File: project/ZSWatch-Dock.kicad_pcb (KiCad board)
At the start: 2 copper layers, 52 x 52 mm, 44 parts, among them IC1 XC9265C181MR-G, IC2 MIC5219-3.3YM5, IC3 NTS0104GU12, IC4 STM32F072CBT6, Q1 BSH205G2AR, SW2 CHARGE, X1 WATCH, X3 DEBUG, X4 USB4105-GF-A

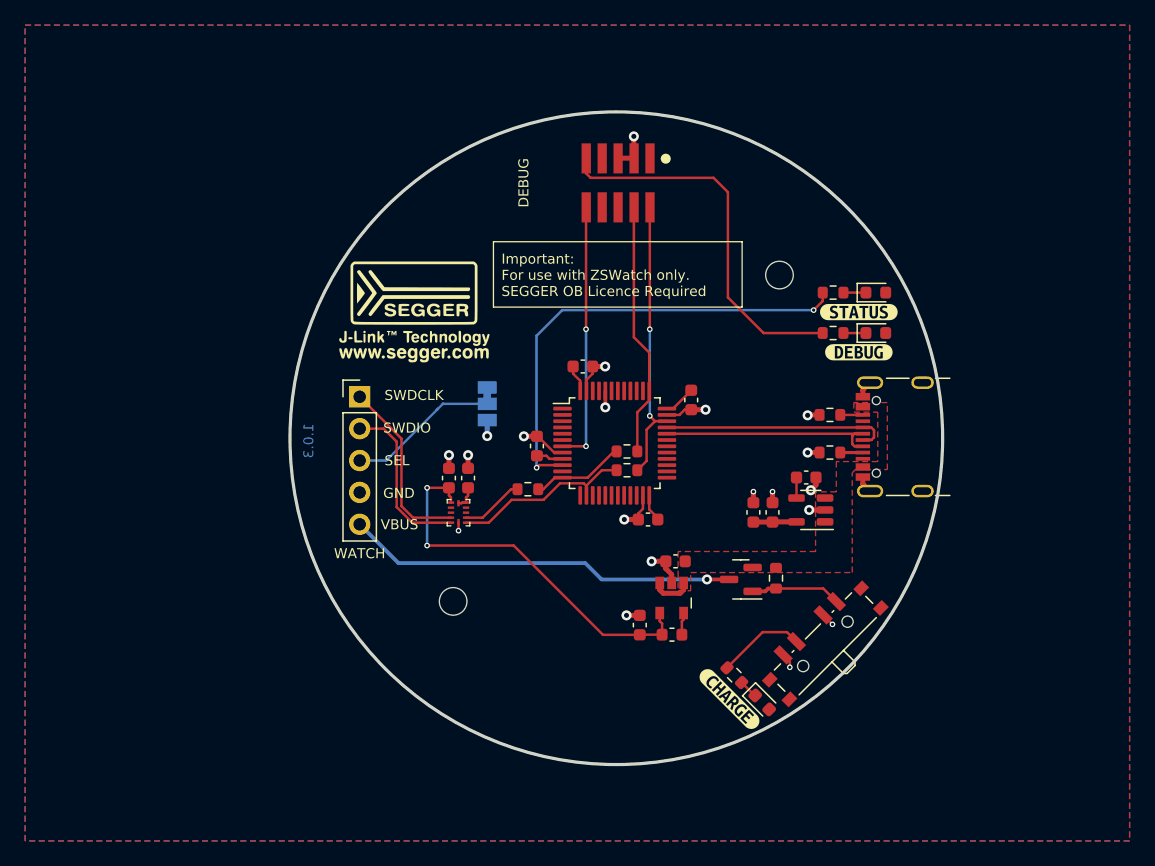
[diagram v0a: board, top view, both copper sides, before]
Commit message: Add second USB interface, rename variants
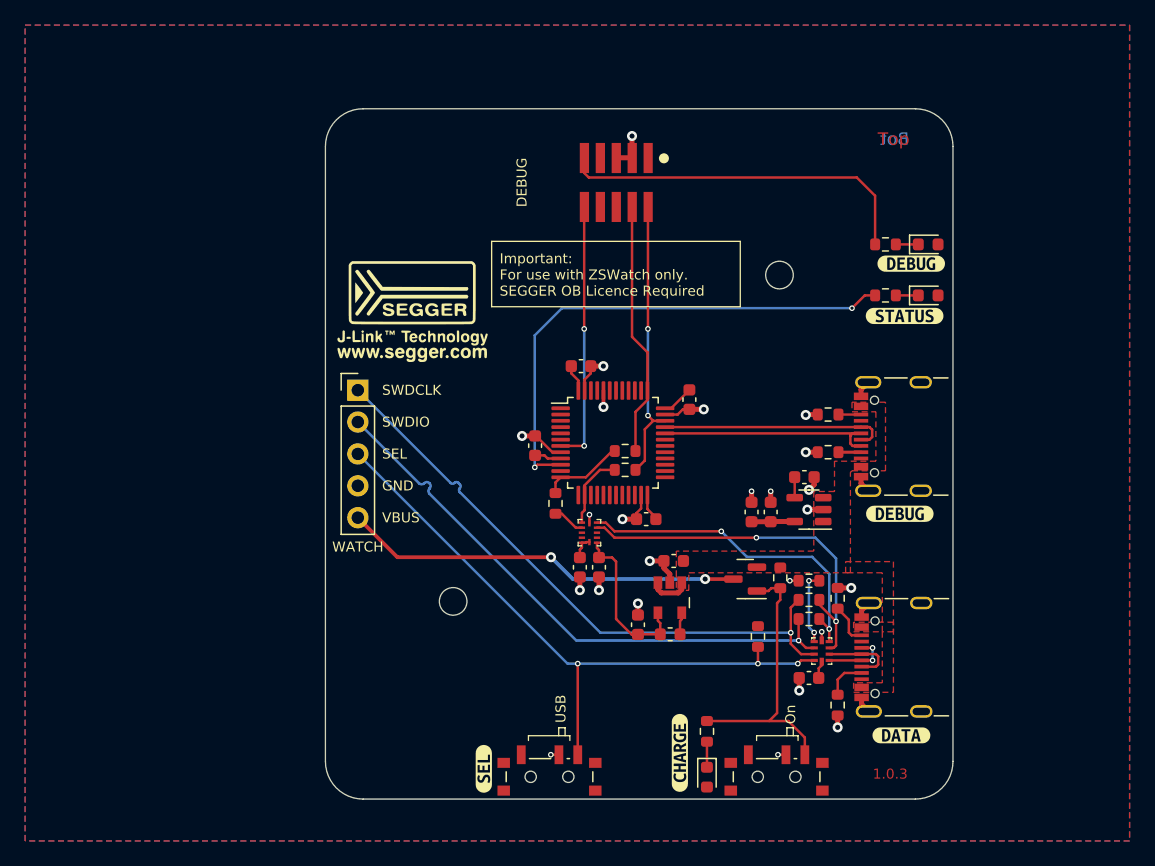
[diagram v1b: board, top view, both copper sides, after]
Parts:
- removed JP1: SEL, Jumper:SolderJumper-3_P1.3mm_Bridged12_Pad1.0x1.5mm_NumberLabels
- added C3: 100n, Capacitor_SMD:C_0603_1608Metric, F.Cu at (169.5, 119.4)
- added IC2: TS3USB221A, Package_QFN:UQFN-10_1.55x2.05mm_P0.5mm, F.Cu at (170.5, 117.2)
- added R1: 100k, Resistor_SMD:R_0603_1608Metric, F.Cu at (165.5, 116.0)
- added R14: 5k1, Resistor_SMD:R_0603_1608Metric, F.Cu at (171.8, 121.5)
- added R15: 5k1, Resistor_SMD:R_0603_1608Metric, F.Cu at (171.8, 113.0)
- added R3: 100k, Resistor_SMD:R_0603_1608Metric, F.Cu at (169.5, 111.6)
- added R4: 0R, Resistor_SMD:R_0603_1608Metric, F.Cu at (169.5, 114.7)
- added R5: 0R, Resistor_SMD:R_0603_1608Metric, F.Cu at (169.5, 113.1)
- added SW2: SEL, Button_Switch_SMD:SW_SPDT_PCM12, F.Cu at (148.9, 126.9)
- added X4: DATA, Connector_USB:USB_C_Receptacle_GCT_USB4105-xx-A_16P_TopMnt_Horizontal, F.Cu at (177.4, 117.7)
- added kibuzzard-65B41384: G***, kibuzzard-65B41384, F.Cu at (176.8, 106.3)
- added kibuzzard-65B413A8: G***, kibuzzard-65B413A8, F.Cu at (143.6, 126.6)
- added kibuzzard-65B413B7: G***, kibuzzard-65B413B7, F.Cu at (176.9, 123.9)
- SW1: renamed from SW2; footprint Button_Switch_SMD:SW_SP3T_PCM13 -> Button_Switch_SMD:SW_SPDT_PCM12
- X3: renamed from X4; value USB4105-GF-A -> DEBUG
- moved C6 13.9 mm to (152.8, 110.5), turned to -90 degrees
- moved C8 11.4 mm to (151.3, 110.5), turned to -90 degrees
- moved SW1 11.1 mm to (166.9, 126.9), turned to 0 degrees
- moved IC4 10.6 mm to (152.0, 107.8), turned to 180 degrees
- moved R10 8.20 mm to (175.6, 84.8)
- moved D2 8.20 mm to (179.0, 84.8)
- moved kibuzzard-6522ABCA 8.20 mm to (177.7, 86.3)
- moved D3 7.40 mm to (161.4, 127.3), turned to -90 degrees
- moved kibuzzard-6525026C 5.83 mm to (159.2, 125.3), turned to 90 degrees
- moved R11 4.98 mm to (161.4, 123.6), turned to 90 degrees
- moved R9 4.18 mm to (175.6, 88.9)
- moved D1 4.18 mm to (179.0, 88.9)
- moved kibuzzard-6522ABB2 3.66 mm to (177.1, 90.5)
- moved G*** 2.52 mm to (156.0, 84.0)
- moved R6 2.48 mm to (149.3, 105.4), turned to 90 degrees
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- renumbered C9 to C10, C10 to C11, C11 to C12, C3 to C4, C4 to C5, C5 to C6, C6 to C7, C7 to C8, C8 to C9, IC2 to IC3, IC3 to IC4, IC4 to IC5, R2 to R10, R10 to R11, R7 to R12, R8 to R13, R9 to R2, R3 to R6, R4 to R7, R5 to R8, R1 to R9, X3 to X2
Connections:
- net USB_DATA_N renamed USB1_DATA_N
- net USB_DATA_P renamed USB1_DATA_P
- IC4 pad 4: ZSWatch_SWDCLK -> SWDCLK_WATCH
- IC4 pad 5: ZSWatch_SWDIO -> SWDIO_WATCH
- Q1 pad 1: Net-(Q1-G) -> CHARGE
- R2 pad 1: Net-(Q1-G) -> CHARGE
- SW1 pad 1: GND -> unconnected-(SW1A-A-Pad1)
- SW1 pad 2: CHARGE -> GND
- SW1 pad 3: GND -> CHARGE
- X1 pad 1: ZSWatch_SWDCLK -> D+/SWDCLK
- X1 pad 2: ZSWatch_SWDIO -> D-/SWDIO
- X1 pad 3: Net-(JP1-C) -> SEL_SWD
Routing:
- net SEL_SWD: track 0.00 -> 52.0 mm, vias 0 -> 3
- net D+/SWDCLK: track 0.00 -> 48.9 mm, vias 0 -> 1
- net D-/SWDIO: track 0.00 -> 46.2 mm, vias 0 -> 1
- net SWDCLK_WATCH: track 0.00 -> 29.9 mm, vias 0 -> 2
- net SWDIO_WATCH: track 0.00 -> 26.7 mm, vias 0 -> 2
- net +1V8: track 31.1 -> 13.2 mm, vias 2 -> 0
- net CHARGE: track 7.02 -> 22.7 mm
- net ZSWatch_SWDCLK: track 14.4 -> 0.00 mm
- net ZSWatch_SWDIO: track 13.4 -> 0.00 mm
- net Net-(JP1-C): track 12.1 -> 0.00 mm
- net /SWDIO: track 14.7 -> 5.98 mm
- net Net-(Q1-G): track 7.20 -> 0.00 mm
- net USB2_DATA_N: track 0.00 -> 6.02 mm
- net GND: track 35.7 -> 41.7 mm, vias 19 -> 24
- net Net-(IC2-~{OE}): track 0.00 -> 5.81 mm, vias 0 -> 2
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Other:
- board size 52 x 52 mm -> 50 x 55 mm
- board text added: "1.0.${REVISION}"
- board text added: "50,0000 mm x 55,0000 mm"
- board text added: "Bot"
- board text added: "On"
- board text added: "Top"
- board text removed: "1.0.3"
- board text removed: "52,0000 mm x 52,0000 mm"
- board text removed: "SWD"
